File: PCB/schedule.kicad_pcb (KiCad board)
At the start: 2 copper layers, 46.8 x 65.1 mm, 7 parts, among them SW1 SW_Push, SW2 SW_Push, SW3 SW_Push, SW4 SW_Push, U1 XIAO-RP2040-DIP

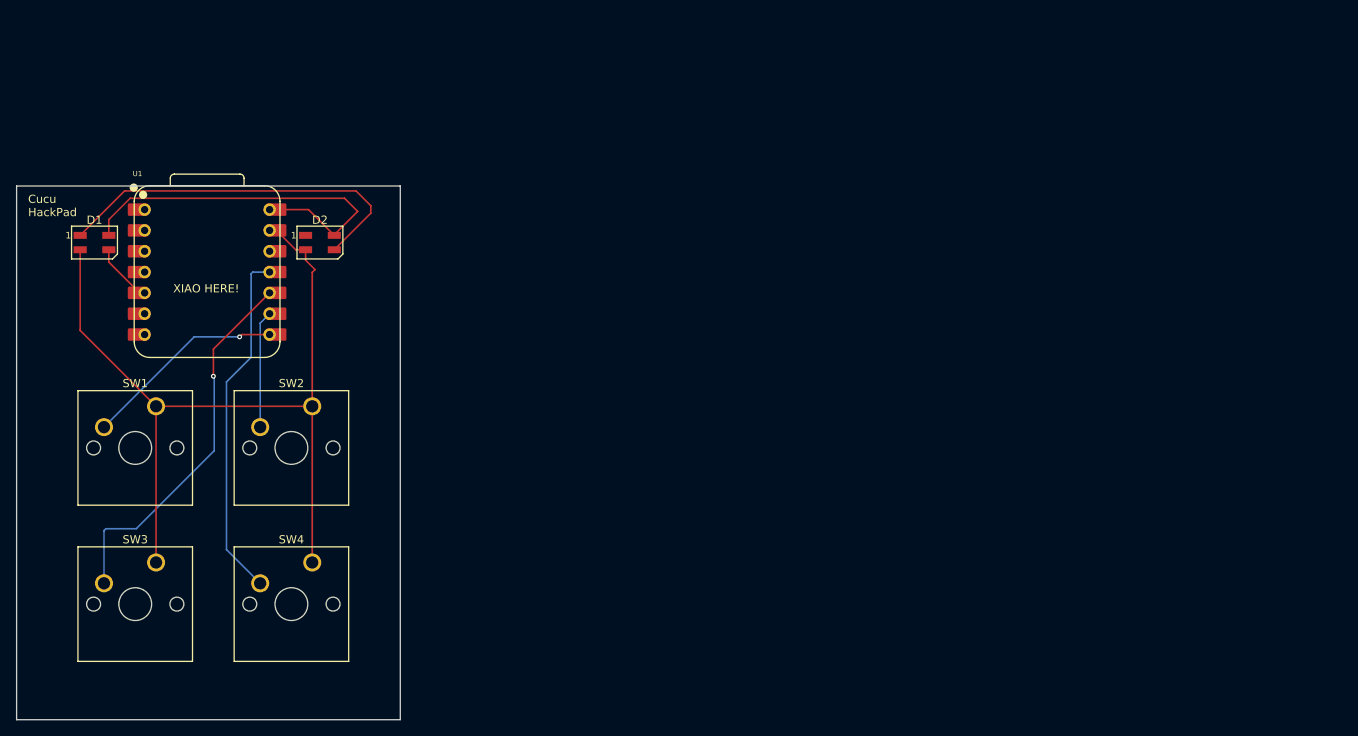
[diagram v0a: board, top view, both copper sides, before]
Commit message: Remodelation
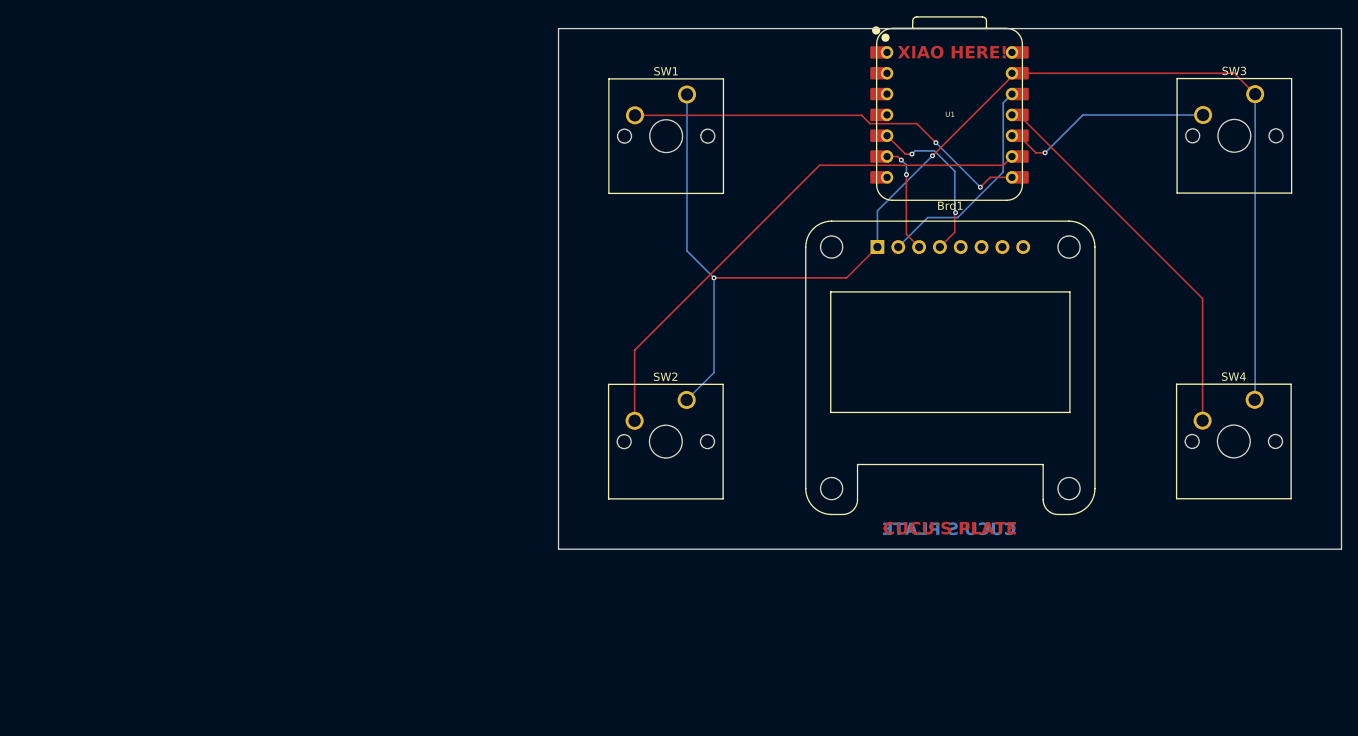
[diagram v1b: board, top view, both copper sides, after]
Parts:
- removed D1, D2: SK6812MINI, LED_SMD:LED_SK6812MINI_PLCC4_3.5x3.5mm_P1.75mm
- added Brd1: SSD1306, Display:Adafruit_SSD1306, F.Cu at (208.9, 63.6)
- moved SW3 145.7 mm to (255.0, 45.0)
- moved SW4 116.6 mm to (254.9, 82.3)
- moved U1 92.6 mm to (217.7, 47.5)
- moved SW1 75.1 mm to (185.7, 45.0)
- moved SW2 45.7 mm to (185.6, 82.3)
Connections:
- U1 pad 12: unconnected-(U1-3V3-Pad12) -> Net-(Brd1-VCC)
- U1 pad 14: +5V -> unconnected-(U1-VBUS-Pad14)
- U1 pad 6: unconnected-(U1-GPIO7/SCL-Pad6) -> Net-(Brd1-SCL)
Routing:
- net GND: track 104.3 -> 156.7 mm, vias 0 -> 2
- net Net-(U1-GPIO2/SCK): track 14.3 -> 64.4 mm
- net +5V: track 47.3 -> 0.00 mm
- net Net-(D1-DOUT): track 45.7 -> 0.00 mm
- net Net-(Brd1-VCC): track 0.00 -> 26.5 mm
- net Net-(U1-GPIO1/RX): track 24.9 -> 50.1 mm, vias 1 -> 2
- net Net-(U1-GPIO4/MISO): track 46.1 -> 25.2 mm
- net Net-(Brd1-SCL): track 0.00 -> 13.4 mm, vias 0 -> 2
- net Net-(Brd1-SDA): track 7.43 -> 20.5 mm, vias 0 -> 2
- net Net-(U1-GPIO3/MOSI): track 43.0 -> 46.6 mm
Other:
- board size 46.8 x 65.1 mm -> 95.5 x 63.5 mm
- board text added: "CUCU'S PLATE"
- board text removed: "Cucu HackPad"
